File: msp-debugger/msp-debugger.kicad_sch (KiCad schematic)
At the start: 13 parts, among them J1 USB_B_Mini, J2 Conn_02x10, SW1 SW_MEC_5E, SW2 SW_MEC_5E, SW3 SW_MEC_5E, SW4 SW_MEC_5E, SW5 SW_Push_Open_Dual, U1 ESP32-S2-SOLO, U2 NHD-0420H1Z

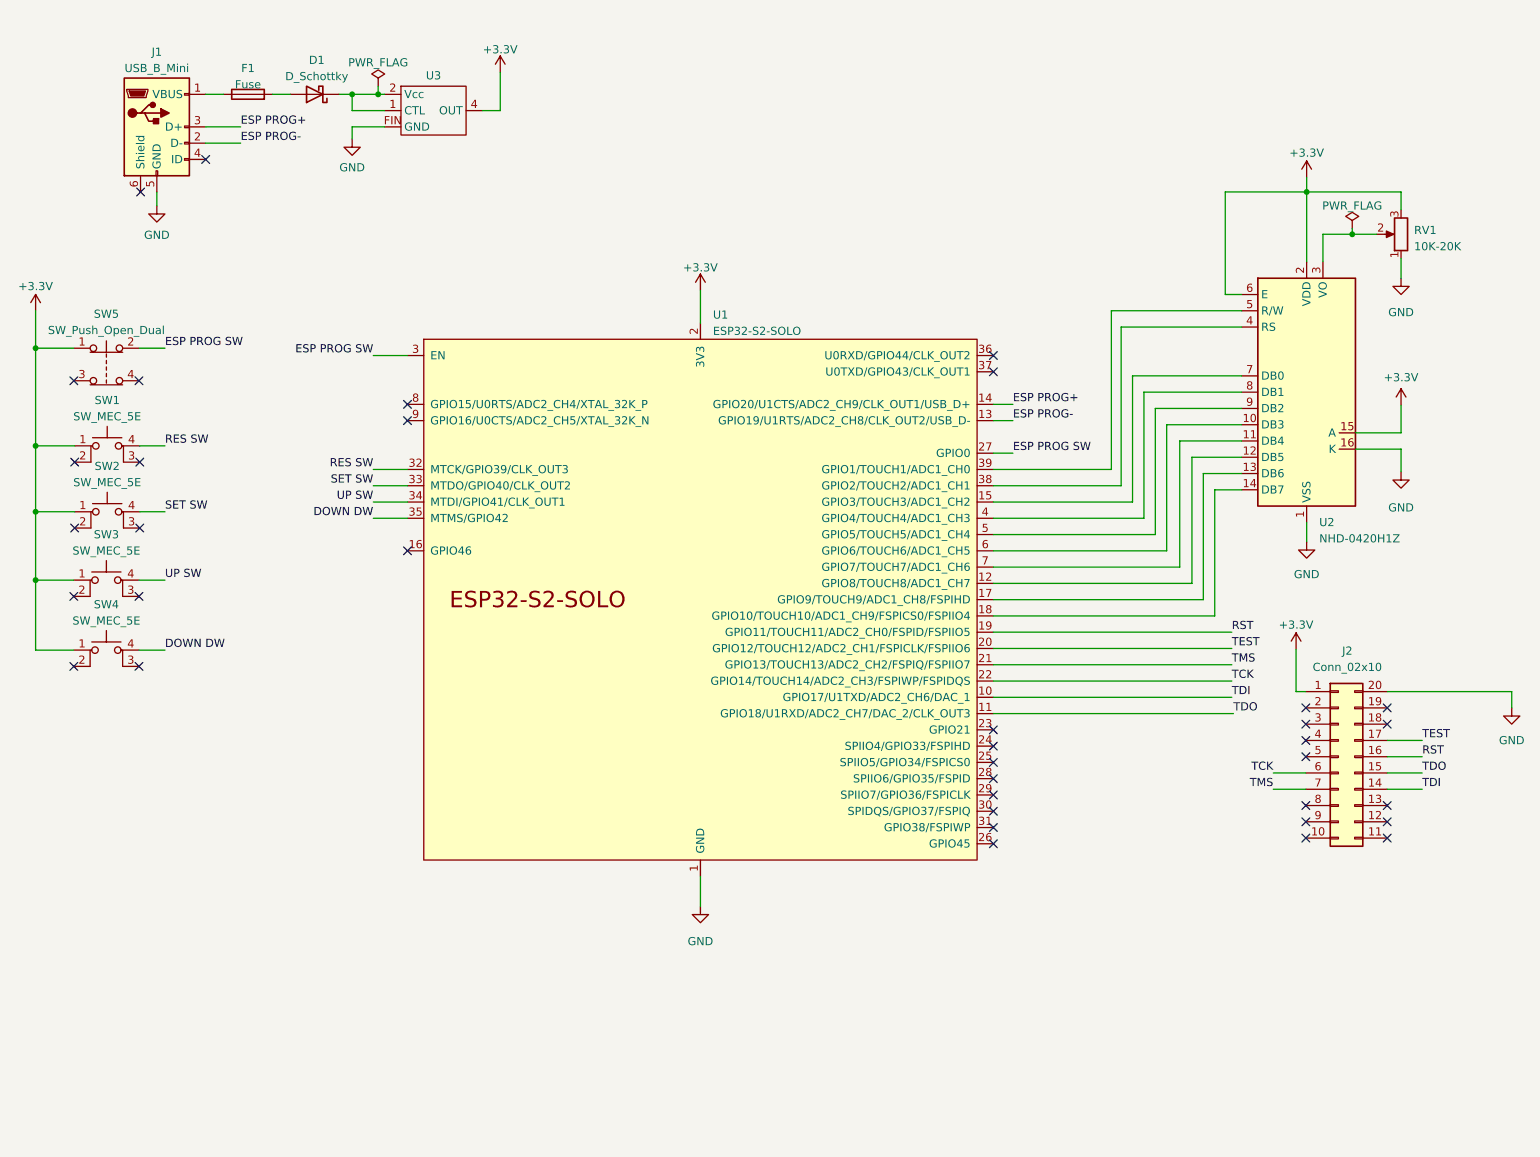
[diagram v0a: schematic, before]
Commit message: finalize schematic
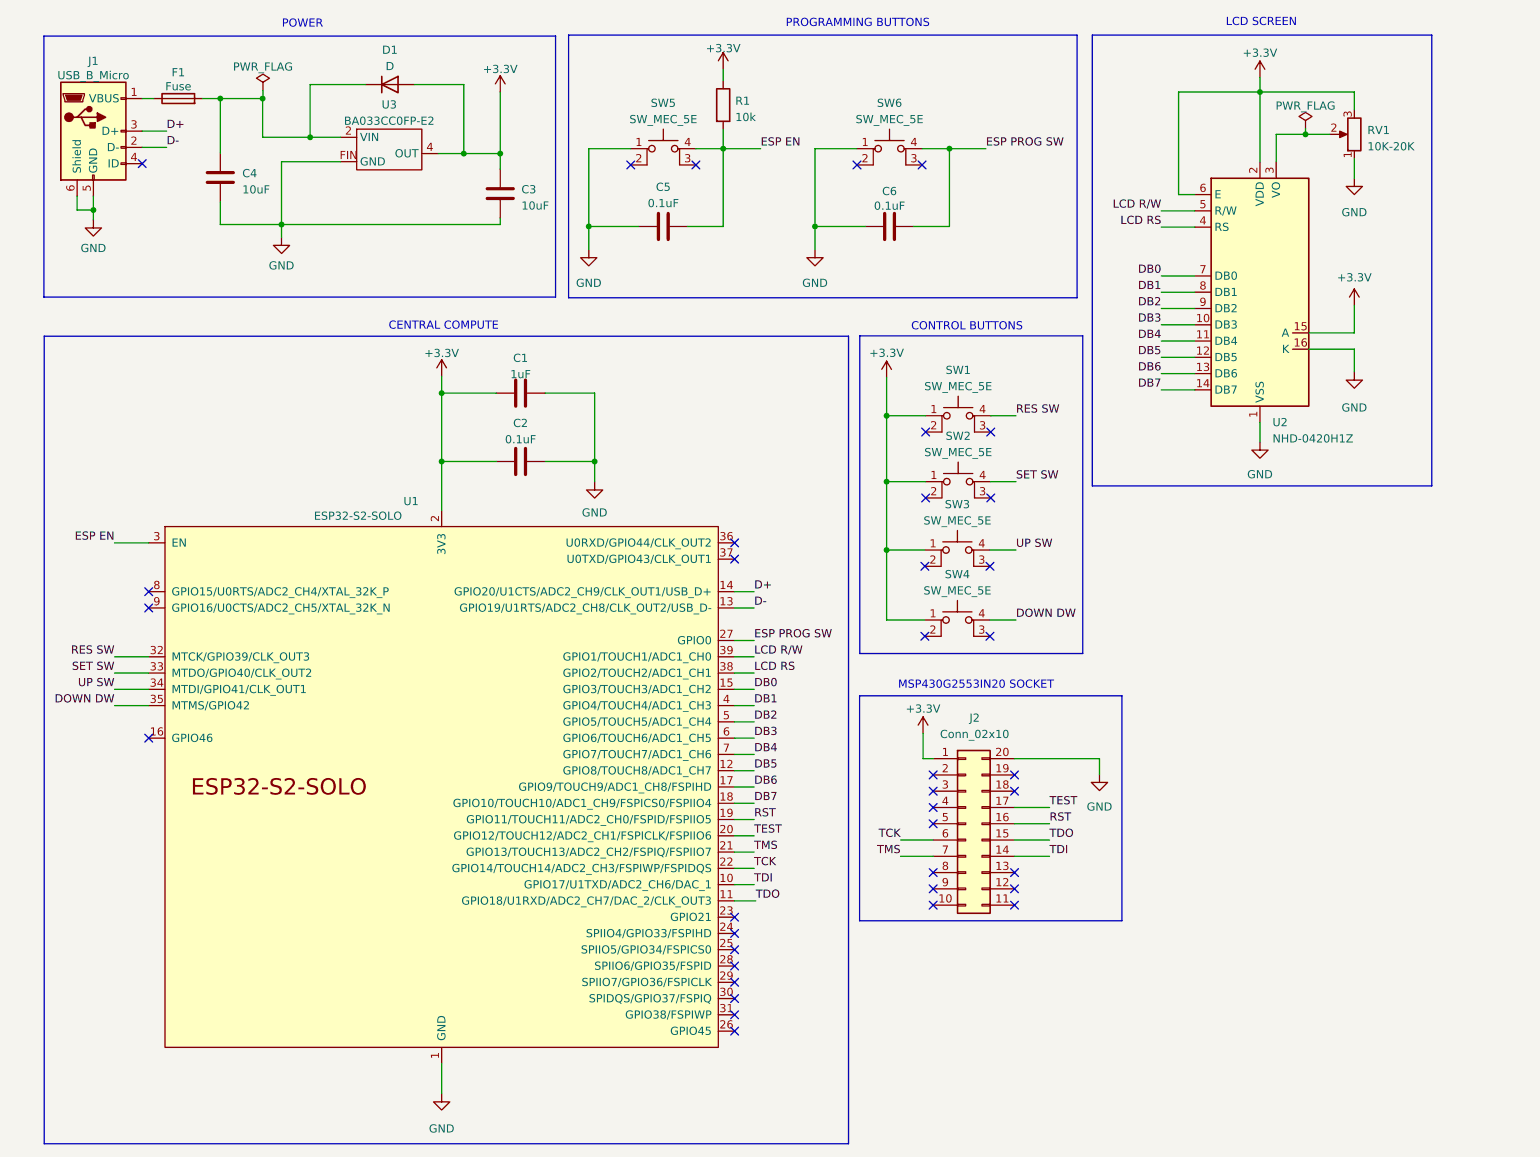
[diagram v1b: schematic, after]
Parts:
- removed D1: D_Schottky, Diode_SMD:D_SOD-128, symbol Device:D_Schottky
- removed J1: USB_B_Mini, symbol Connector:USB_B_Mini
- removed SW5: SW_Push_Open_Dual, symbol Switch:SW_Push_Open_Dual
- added C1: 1uF, symbol Device:C
- added C2, C5, C6: 0.1uF, symbol Device:C
- added C3, C4: 10uF, symbol Device:C
- added D1: D, symbol Device:D
- added J1: USB_B_Micro, symbol Connector:USB_B_Micro
- added R1: 10k, symbol Device:R
- added SW5, SW6: SW_MEC_5E, symbol Switch:SW_MEC_5E
- U3: value ~ -> BA033CC0FP-E2
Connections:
- net +3.3V: now also C1.1, C2.1, C3.1, D1.2 (A), R1.1
- net ESP PROG SW: now also C6.1, SW6.4 (A); no longer U1.3 (EN)
- net GND: now also C1.2, C2.2, C3.2, C4.2, C5.2, C6.2, J1.5 (GND), J1.6 (Shield), SW5.1, SW6.1
- net DB3: now reaches U1.6 (GPIO6/TOUCH6/ADC1_CH5), U2.10 (DB3)
- net DB4: now reaches U1.7 (GPIO7/TOUCH7/ADC1_CH6), U2.11 (DB4)
- net DB5: now reaches U1.12 (GPIO8/TOUCH8/ADC1_CH7), U2.12 (DB5)
- net DB6: now reaches U1.17 (GPIO9/TOUCH9/ADC1_CH8/FSPIHD), U2.13 (DB6)
- net DB7: now reaches U1.18 (GPIO10/TOUCH10/ADC1_CH9/FSPICS0/FSPIIO4), U2.14 (DB7)
- net LCD RS: now reaches U1.38 (GPIO2/TOUCH2/ADC1_CH1), U2.4 (RS)
- net LCD R/W: now reaches U1.39 (GPIO1/TOUCH1/ADC1_CH0), U2.5 (R/W)
- net DB0: now reaches U1.15 (GPIO3/TOUCH3/ADC1_CH2), U2.7 (DB0)
- net DB1: now reaches U1.4 (GPIO4/TOUCH4/ADC1_CH3), U2.8 (DB1)
- net DB2: now reaches U1.5 (GPIO5/TOUCH5/ADC1_CH4), U2.9 (DB2)
- net at U3.2 (VIN): now also F1.2, C4.1, D1.1 (K); no longer U3.1 (CTL)
- net at F1.1: now also J1.1 (VBUS)
- net ESP PROG+ renamed D+
- net D+: now also J1.3 (D+)
- net ESP PROG- renamed D-
- net D-: now also J1.2 (D-)
- new net ESP EN: C5.1, R1.2, SW5.4 (A), U1.3 (EN)
- no-connect marks 37 -> 38
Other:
- note added: "CENTRAL COMPUTE"
- note added: "CONTROL BUTTONS"
- note added: "LCD SCREEN"
- note added: "MSP430G2553IN20 SOCKET"
- note added: "POWER"
- note added: "PROGRAMMING BUTTONS"
- moved on the sheet: F1, J2, RV1, SW1, SW2, SW3, SW4, U1, U2
